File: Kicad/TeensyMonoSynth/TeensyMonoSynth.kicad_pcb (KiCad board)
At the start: 2 copper layers, 162 x 110 mm, 22 parts, among them U1 74HCT4051, U2 74HCT4051, U3 74HCT4051

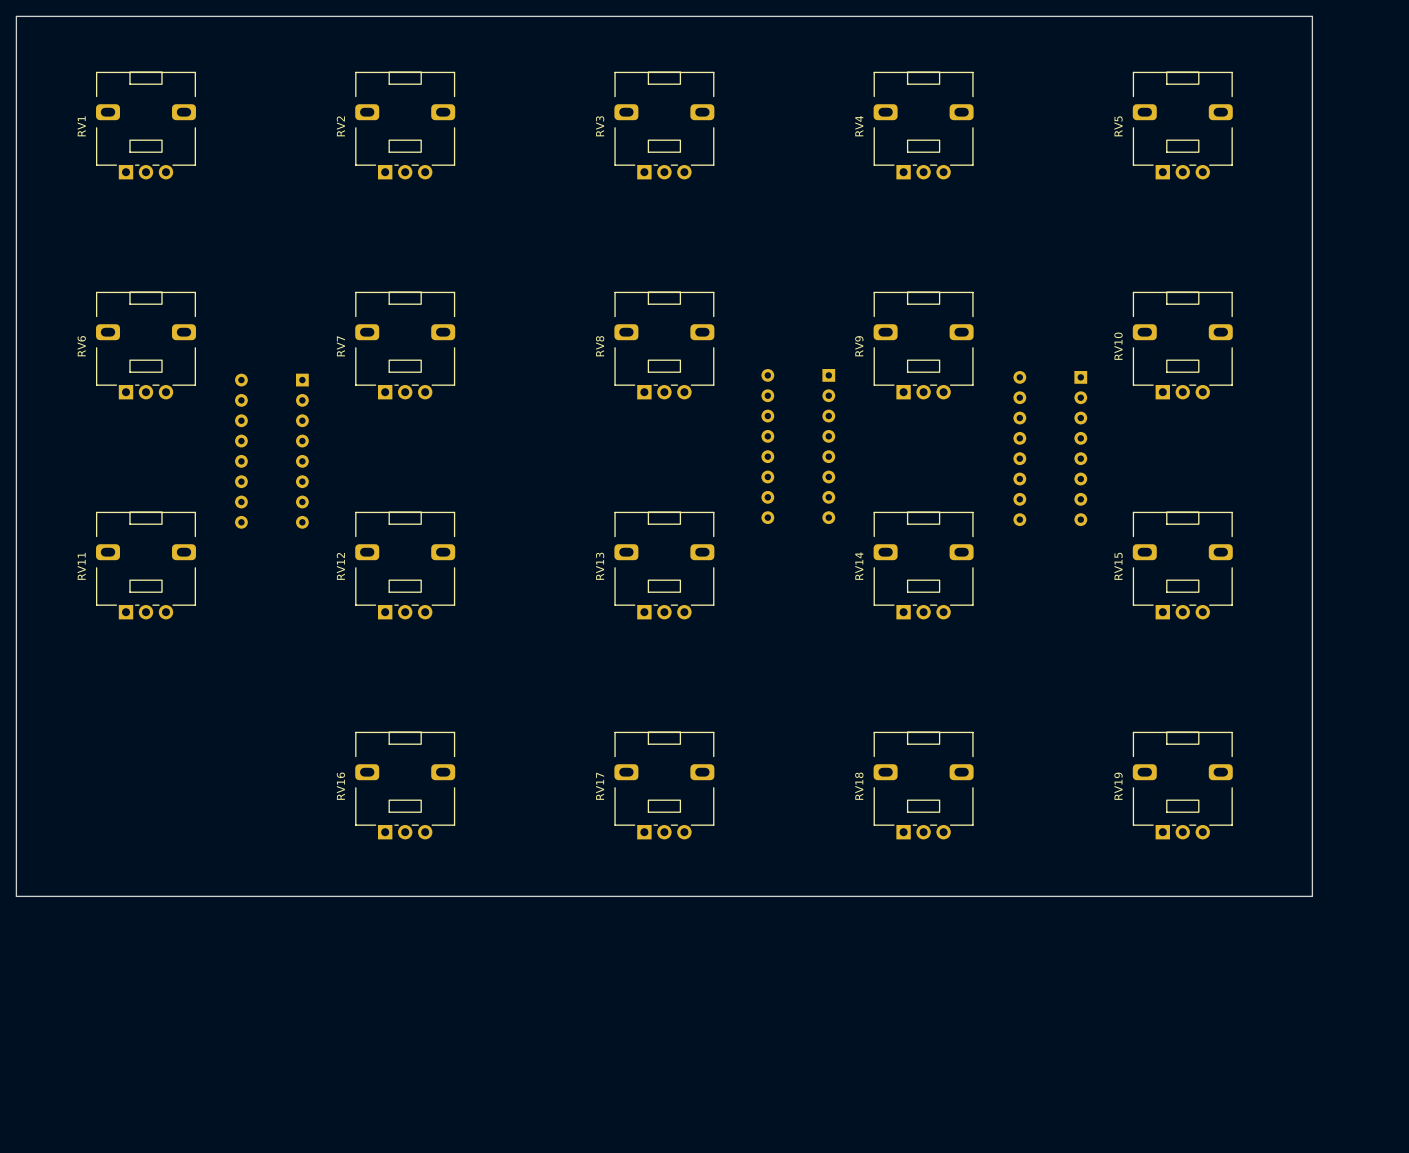
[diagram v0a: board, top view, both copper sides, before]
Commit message: PCB LAYOUT COMPLETE
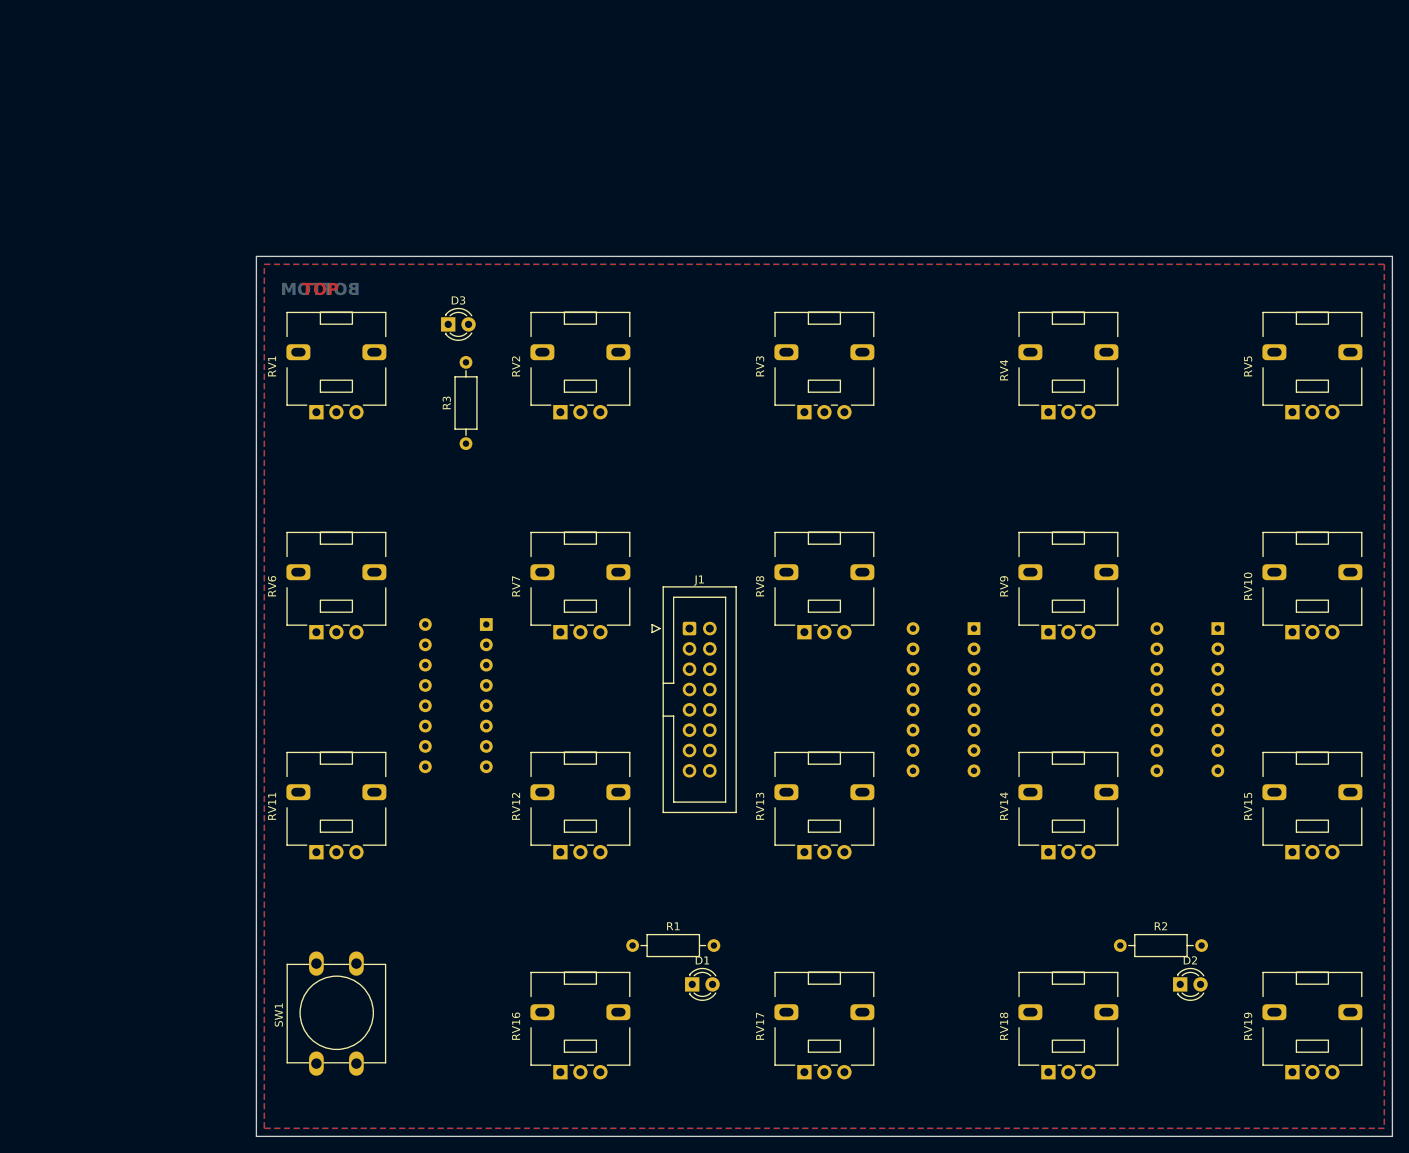
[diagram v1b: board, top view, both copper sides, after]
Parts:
- added D1: LED, LED_THT:LED_D3.0mm, F.Cu at (104.5, 141.0)
- added D2: LED, LED_THT:LED_D3.0mm, F.Cu at (165.5, 141.0)
- added D3: LED, LED_THT:LED_D3.0mm, F.Cu at (74.0, 58.5)
- added J1: Conn_01x16_Socket, Connector_IDC:IDC-Header_2x08_P2.54mm_Vertical, F.Cu at (104.1, 96.5)
- added R1: R, Resistor_THT:R_Axial_DIN0207_L6.3mm_D2.5mm_P10.16mm_Horizontal, F.Cu at (97.0, 136.1)
- added R2: R, Resistor_THT:R_Axial_DIN0207_L6.3mm_D2.5mm_P10.16mm_Horizontal, F.Cu at (158.0, 136.1)
- added R3: R, Resistor_THT:R_Axial_DIN0207_L6.3mm_D2.5mm_P10.16mm_Horizontal, F.Cu at (76.2, 73.4)
- added SW1: SW_Push, Button_Switch_THT:SW_PUSH-12mm, F.Cu at (57.5, 150.9)
- moved RV1 38.3 mm to (57.5, 69.5)
- moved RV11 38.3 mm to (57.5, 124.5)
- moved RV6 38.3 mm to (57.5, 97.0)
- moved U1 38.2 mm to (78.7, 96.0)
- moved RV12 37.1 mm to (88.0, 124.5)
- moved RV16 37.1 mm to (88.0, 152.0)
- moved RV2 37.1 mm to (88.0, 69.5)
- moved RV7 37.1 mm to (88.0, 97.0)
- moved U2 36.5 mm to (139.7, 96.5)
- moved RV13 36.1 mm to (118.5, 124.5)
- moved RV17 36.1 mm to (118.5, 152.0)
- moved RV8 36.1 mm to (118.5, 97.0)
- moved RV3 36.1 mm to (118.5, 69.5)
- moved U3 35.8 mm to (170.2, 96.5)
- moved RV14 35.0 mm to (149.0, 124.5)
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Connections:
- U1 pad 3: unconnected-(U1-A-Pad3) -> SIG_MUX1
- U2 pad 3: unconnected-(U2-A-Pad3) -> SIG_MUX2
- U3 pad 3: unconnected-(U3-A-Pad3) -> SIG_MUX3
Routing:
- added copper zone on In2.Cu, net +3.3V
- added copper zone on B.Cu, net GND
- added copper zone on F.Cu, net GND
- added copper zone on In1.Cu, net GND
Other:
- board size 162 x 110 mm -> 142 x 110 mm
- copper layers 2 -> 4
- board text added: "BOTTOM"
- board text added: "INNER 1"
- board text added: "INNER 2"
- board text added: "TOP"
